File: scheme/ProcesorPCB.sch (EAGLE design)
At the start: 28 parts, among them U1 UA78L05ACPKG3, X1 22-23-2031, X12 22-23-2051

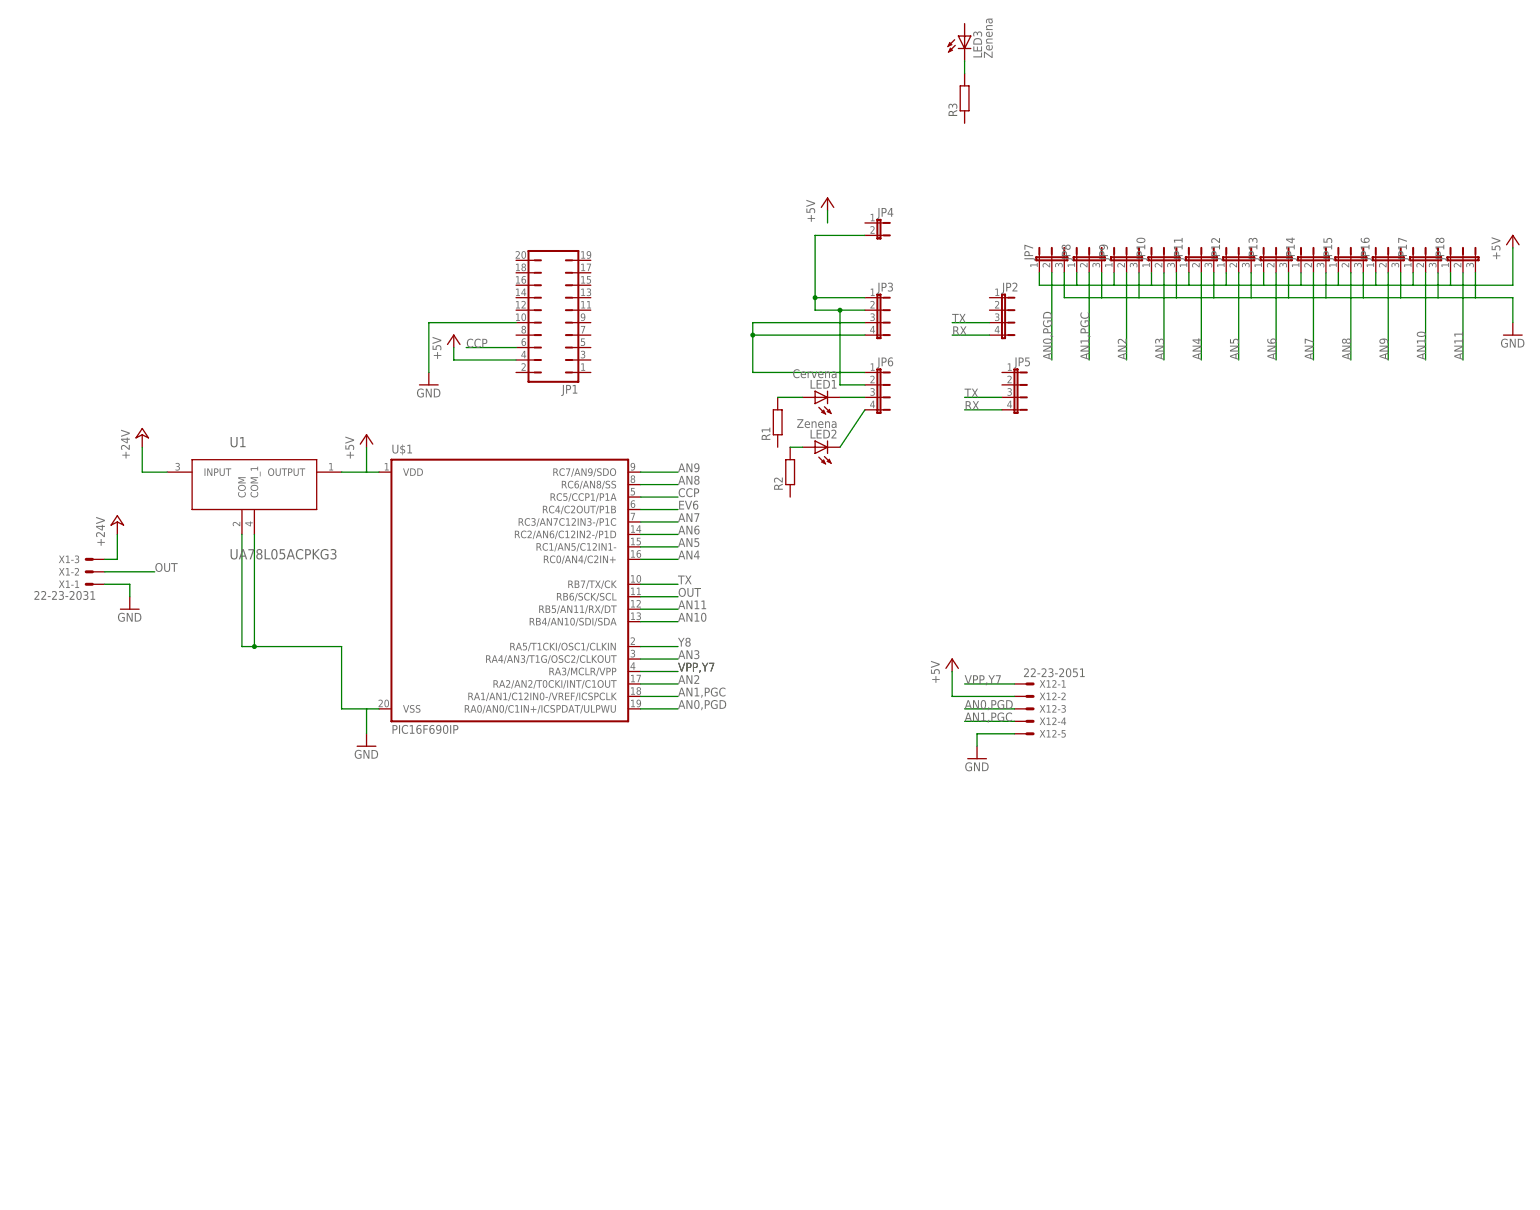
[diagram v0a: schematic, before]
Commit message: PCB borad almost finished.
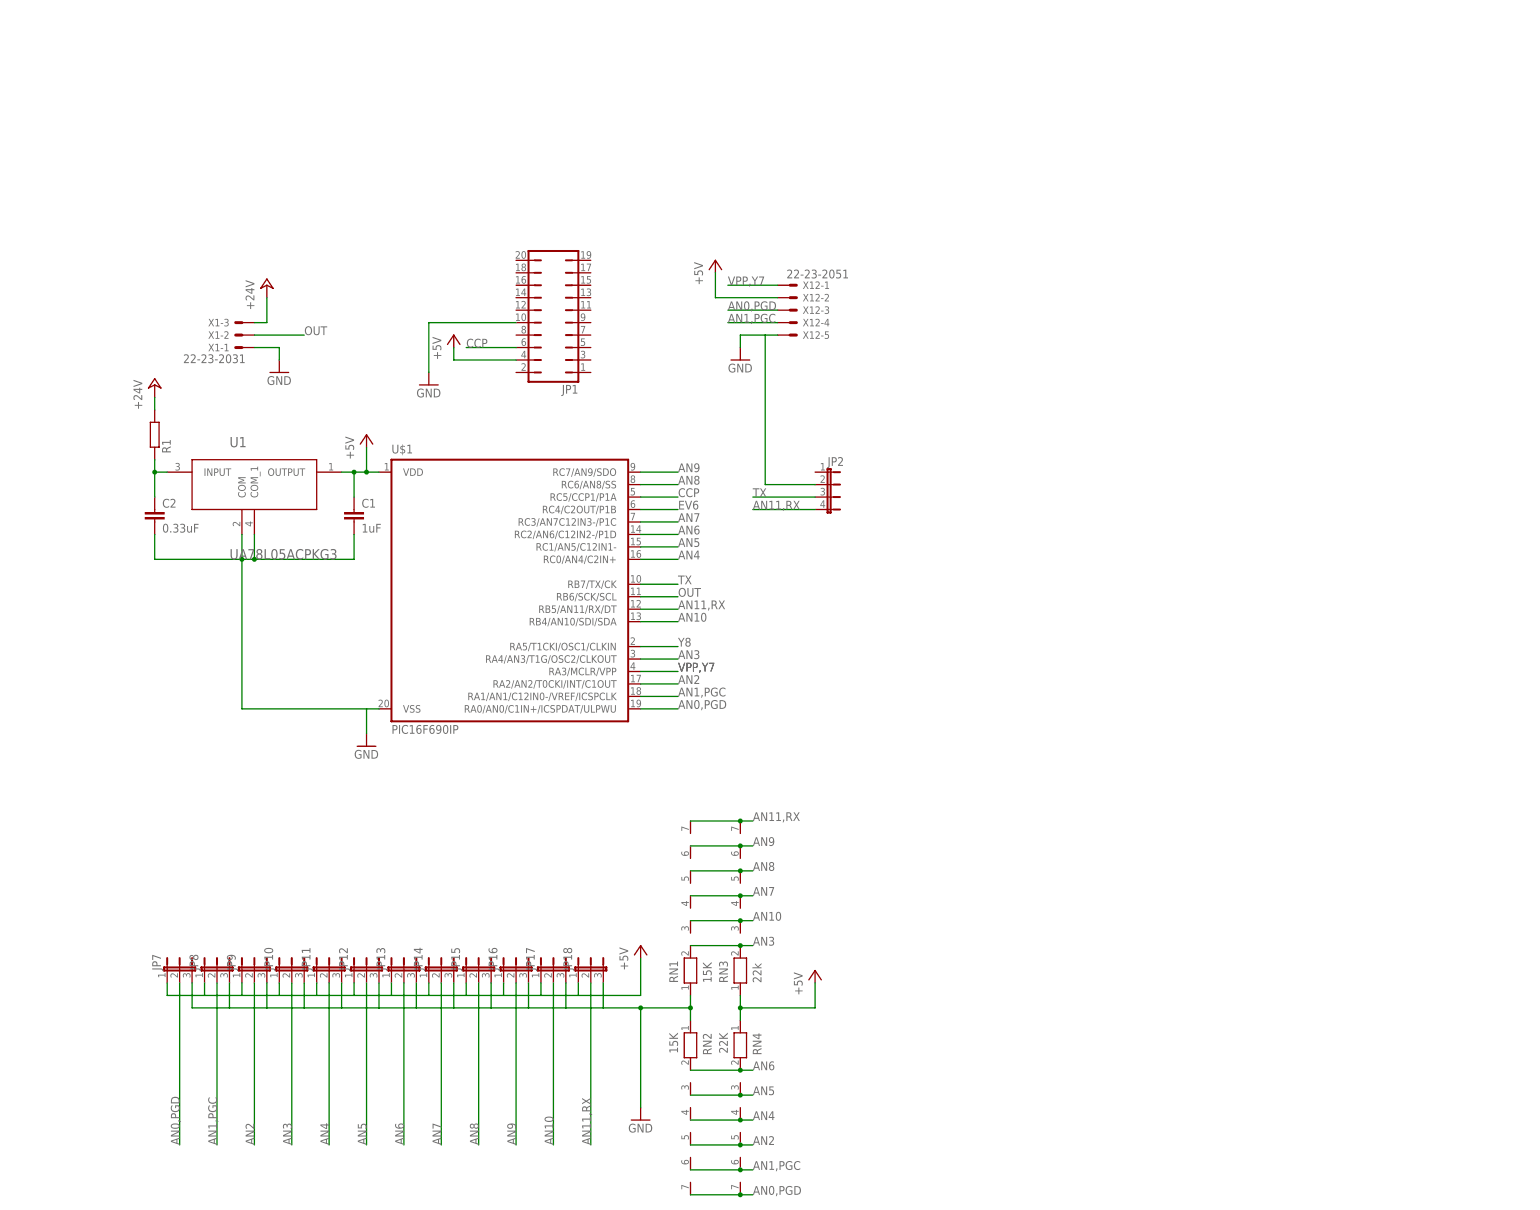
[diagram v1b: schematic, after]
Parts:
- removed JP3, JP5, JP6: (no value), jumper:JP4E
- removed JP4: (no value), jumper:JP1E
- removed LED1: Cervena, led:LED5MM
- removed LED2, LED3: Zenena, led:LED5MM
- removed R2, R3: (no value), rcl:R-EU_R0805W
- added C1: 1uF, resistor:C-EU025-030X050
- added C2: 0.33uF, resistor:C-EU025-030X050
- added RN1, RN2: 15K, resistor-net:RN06
- added RN3: 22k, resistor-net:RN06
- added RN4: 22K, resistor-net:RN06
- R1: device rcl:R-EU_R0805W -> resistor:R-EU_0207/10
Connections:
- removed net AN11: JP18.2, U$1.RB5/AN11/RX/DT
- removed net N$3: JP6.4, LED2.C
- removed net N$4: JP6.3, LED1.C
- removed net N$5: LED2.A, R2.2
- removed net N$6: LED1.A, R1.2
- removed net N$8: LED3.C, R3.2
- removed net N$9: JP3.3, JP3.4, JP6.1
- removed net RX: JP2.4, JP5.4
- new net AN11,RX: JP18.2, JP2.4, RN1.7, RN3.7, U$1.RB5/AN11/RX/DT
- net +24V: now also R1.2; no longer U1.INPUT
- net +5V: now also C1.1, RN3.1, RN4.1
- net AN0,PGD: now also RN2.7, RN4.7
- net AN1,PGC: now also RN2.6, RN4.6
- net AN10: now also RN1.3, RN3.3
- net AN2: now also RN2.5, RN4.5
- net AN3: now also RN1.2, RN3.2
- net AN4: now also RN2.4, RN4.4
- net AN5: now also RN2.3, RN4.3
- net AN6: now also RN2.2, RN4.2
- net AN7: now also RN1.4, RN3.4
- net AN8: now also RN1.5, RN3.5
- net AN9: now also RN1.6, RN3.6
- net GND: now also C1.2, C2.2, JP2.2, RN1.1, RN2.1
- net N$2: now also C2.1, R1.1, U1.INPUT; no longer JP3.1, JP3.2, JP4.2, JP6.2
- net TX: no longer JP5.3
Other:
- moved on the sheet: JP10, JP11, JP12, JP13, JP14, JP15, JP16, JP17, JP18, JP2, JP7, JP8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
